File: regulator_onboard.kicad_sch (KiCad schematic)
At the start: 12 parts, among them U16 TLV71333PDQN, U18 TPS2116DRL

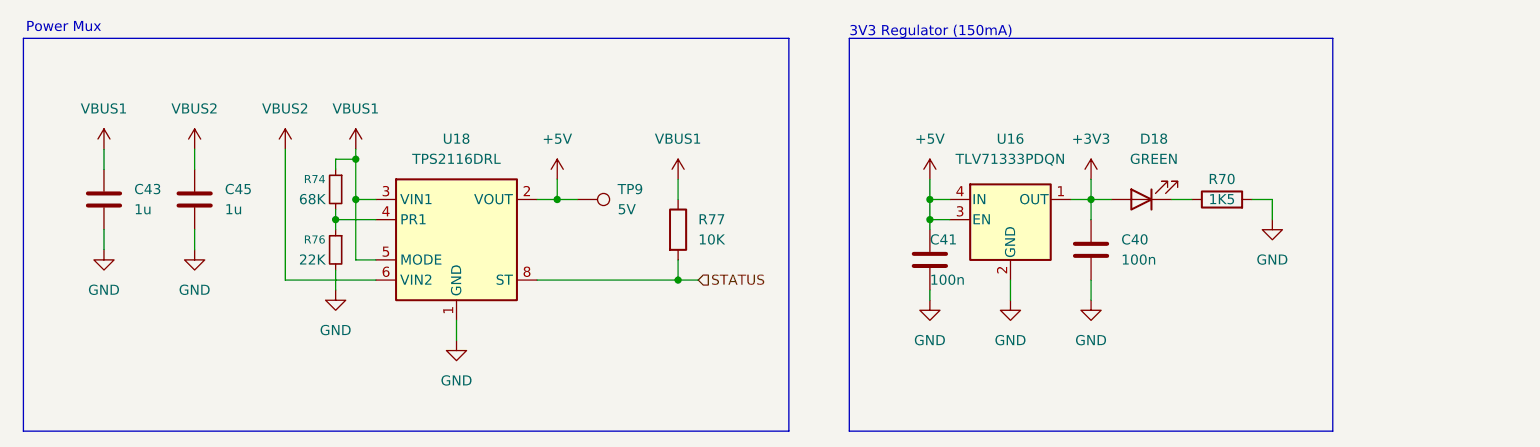
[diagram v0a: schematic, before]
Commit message: finish layout
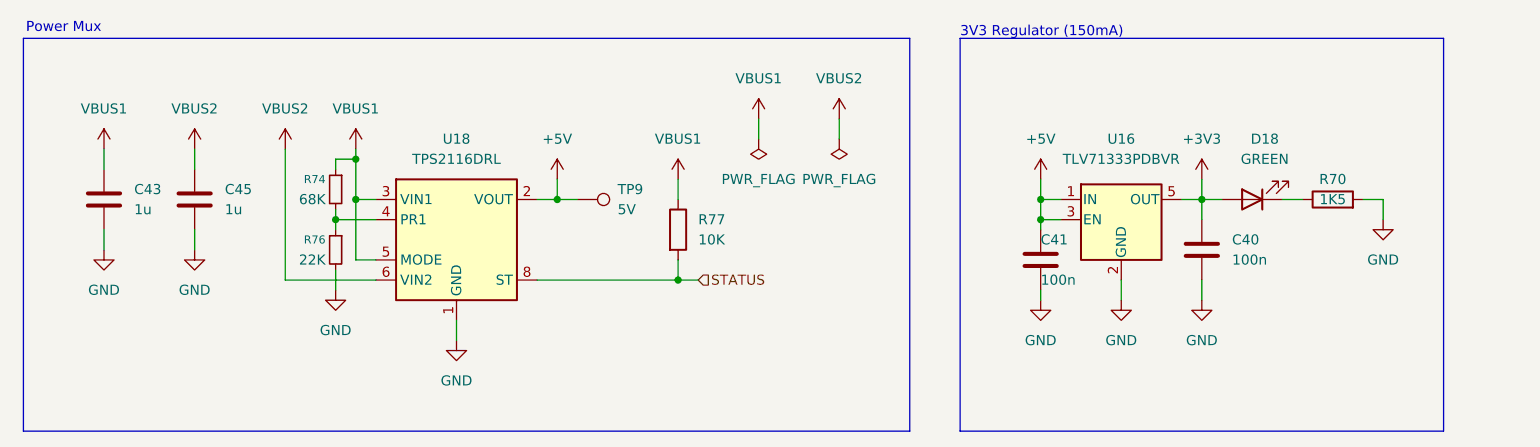
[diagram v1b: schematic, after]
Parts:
- U16: value TLV71333PDQN -> TLV71333PDBVR; symbol TLV71333PDQ:TLV71333PDQN -> TLV71333PDQ:TLV71333PDBVR
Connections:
- net +3V3: now also U16.5 (OUT); no longer U16.1 (OUT)
- net +5V: now also U16.1 (IN); no longer U16.4 (IN)
- net GND: no longer U16.5 (GND)
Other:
- moved on the sheet: C40, C41, D18, R70, U16

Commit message: improvements with derick
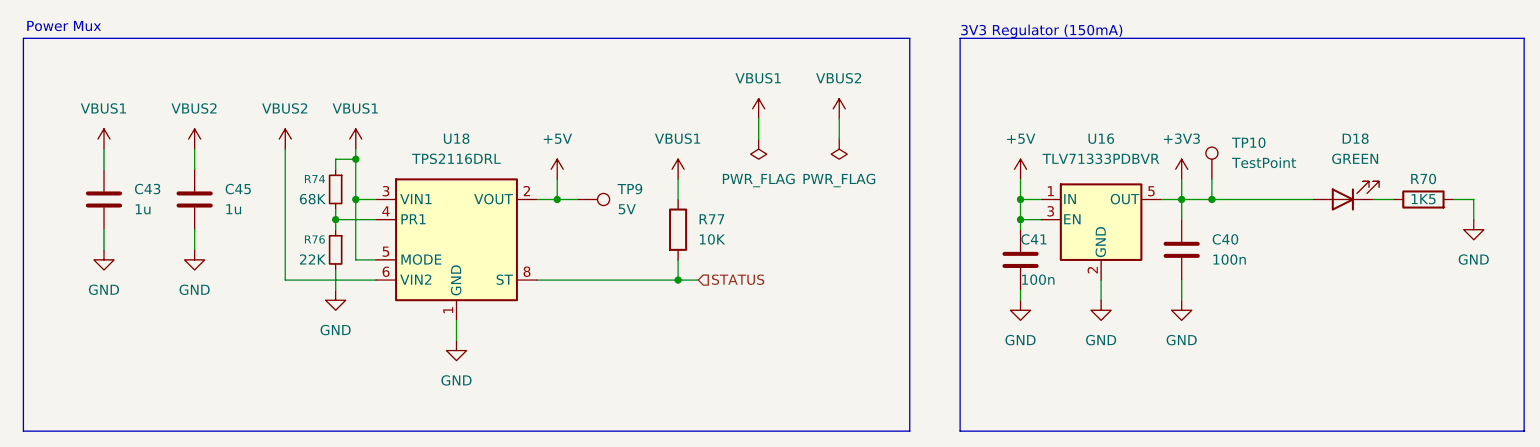
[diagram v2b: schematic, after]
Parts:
- added TP10: TestPoint, TestPoint:TestPoint_Pad_1.0x1.0mm, symbol Connector:TestPoint
- TP9: now left out of the parts list
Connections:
- net +3V3: now also TP10.1
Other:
- moved on the sheet: C40, C41, D18, R70, U16
